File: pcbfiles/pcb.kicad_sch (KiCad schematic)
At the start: 236 parts, among them J1 Conn_01x06, J2 Conn_01x06, J3 Conn_01x06, J4 Conn_01x06, J5 Conn_01x04_Female, J6 Conn_01x04_Female, Q1 AO3401A, Q2 AO3401A, SW1 SW_SPST, SW10 SW_SPST, SW11 SW_SPST, SW12 SW_SPST, SW13 SW_SPST, SW14 SW_SPST, SW15 SW_SPST, SW16 SW_SPST, SW17 SW_SPST, SW18 SW_SPST, SW19 SW_SPST, SW2 SW_SPST, SW20 SW_SPST, SW21 SW_SPST, SW22 SW_SPST, SW23 SW_SPST, SW24 SW_SPST, SW25 SW_SPST, SW26 SW_SPST, SW27 SW_SPST, SW28 SW_SPST, SW29 SW_SPST, SW3 SW_SPST, SW30 SW_SPST, SW31 SW_SPST, SW32 SW_SPST, SW33 SW_SPST, SW34 SW_SPST, SW35 SW_SPST, SW36 SW_SPST, SW37 SW_SPST, SW38 SW_SPST, SW39 SW_SPST, SW4 SW_SPST, SW40 SW_SPST, SW41 SW_SPST, SW42 SW_SPST, SW43 SW_SPST, SW44 SW_SPST, SW45 SW_SPST, SW46 SW_SPST, SW47 SW_SPST, SW48 SW_SPST, SW49 SW_SPST, SW5 SW_SPST, SW50 SW_SPST, SW51 SW_SPST, SW52 SW_SPST, SW53 SW_SPST, SW54 SW_SPST, SW55 SW_SPST, SW56 SW_SPST, SW57 SW_SPST, SW58 SW_SPST, SW59 SW_SPST, SW6 SW_SPST, SW60 SW_SPST, SW61 SW_SPST, SW62 SW_SPST, SW63 SW_SPST, SW64 SW_SPST, SW65 SW_SPST, SW66 SW_SPST, SW67 SW_SPST, SW68 SW_SPST, SW69 SW_SPST, SW7 SW_SPST, SW70 SW_SPST, SW71 SW_SPST, SW72 SW_SPST, SW73 SW_SPST, SW74 SW_SPST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

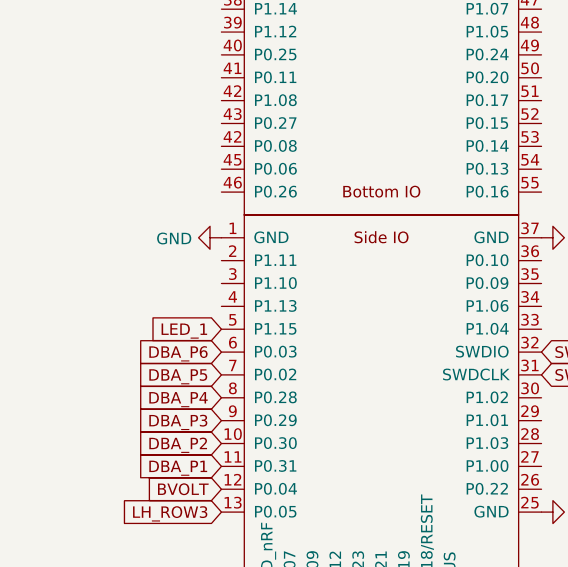
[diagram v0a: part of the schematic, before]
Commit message: Routing progress.
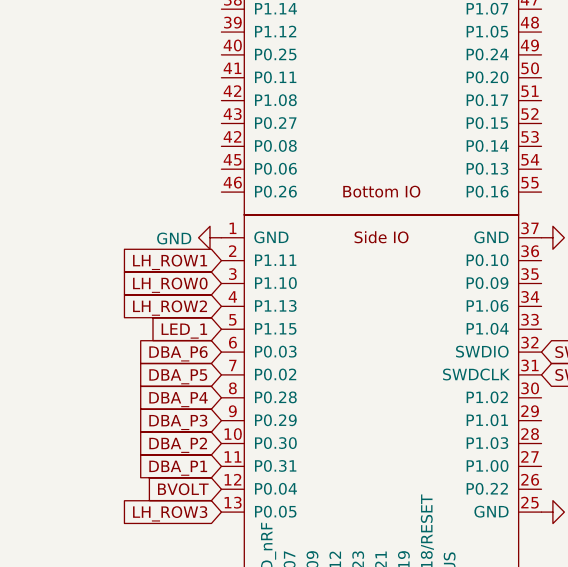
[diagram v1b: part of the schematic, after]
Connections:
- net LH_ROW0: now also U5.3 (P1.10)
- net LH_ROW1: now also U5.2 (P1.11)
- net LH_ROW2: now also U5.4 (P1.13)
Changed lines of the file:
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@@
+    )
+  )
+  (global_label "LH_ROW1" (shape input) (at 36.322 247.65 180) (fields_autoplaced)
+    (effects (font (size 1.27 1.27)) (justify right))
+    (property "Intersheet References" "${INTERSHEET_REFS}" (id 0) (at -90.678 124.46 0)
+      (effects (font (size 1.27 1.27)) hide)
     )
   )
@@
     )
   )
+  (global_label "LH_ROW0" (shape input) (at 36.322 250.19 180) (fields_autoplaced)
+    (effects (font (size 1.27 1.27)) (justify right))
+    (property "Intersheet References" "${INTERSHEET_REFS}" (id 0) (at -90.678 137.16 0)
+      (effects (font (size 1.27 1.27)) hide)
+    )
+  )
   (global_label "ENC_A_B" (shape input) (at 497.84 129.032 180) (fields_autoplaced)
     (effects (font (size 1.27 1.27)) (justify right))
@@
       (effects (font (size 1.27 1.27)) hide)
     )
+  )
+  (global_label "LH_ROW2" (shape input) (at 36.322 252.73 180) (fields_autoplaced)
+    (effects (font (size 1.27 1.27)) (justify right))
+    (property "Intersheet References" "${INTERSHEET_REFS}" (id 0) (at -90.678 119.38 0)
+      (effects (font (size 1.27 1.27)) hide)
+    )

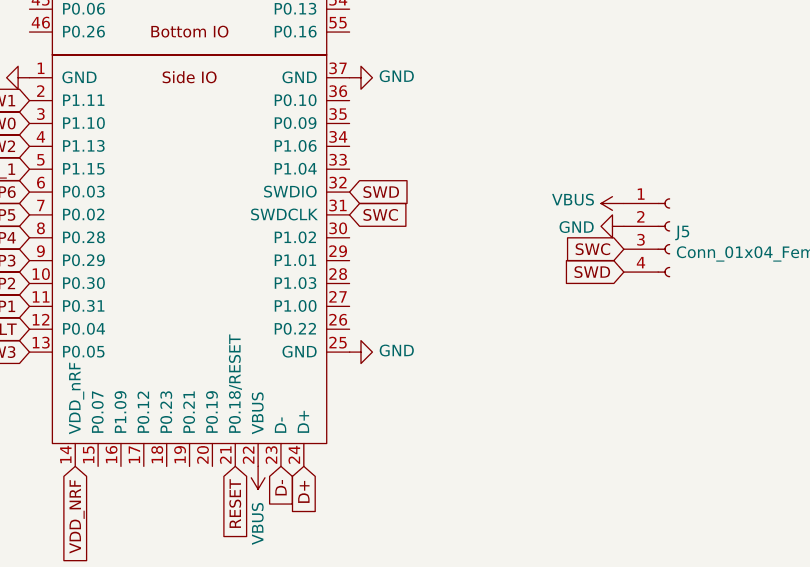
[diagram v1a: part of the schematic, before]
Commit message: practically done with the left half
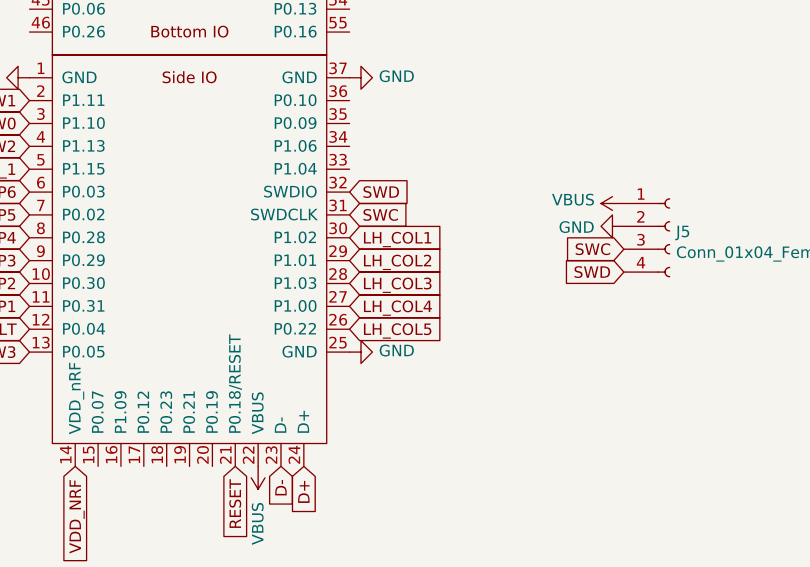
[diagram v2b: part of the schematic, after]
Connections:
- net LH_COL1: now also U5.30 (P1.02)
- net LH_COL2: now also U5.29 (P1.01)
- net LH_COL3: now also U5.28 (P1.03)
- net LH_COL4: now also U5.27 (P1.00)
- net LH_COL5: now also U5.26 (P0.22)
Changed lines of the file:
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@@
+    )
+  )
+  (global_label "LH_COL1" (shape input) (at 71.882 262.89 0) (fields_autoplaced)
+    (effects (font (size 1.27 1.27)) (justify left))
+    (property "Intersheet References" "${INTERSHEET_REFS}" (id 0) (at 169.672 110.49 0)
+      (effects (font (size 1.27 1.27)) hide)
     )
   )
@@
     )
   )
+  (global_label "LH_COL5" (shape input) (at 71.882 273.05 0) (fields_autoplaced)
+    (effects (font (size 1.27 1.27)) (justify left))
+    (property "Intersheet References" "${INTERSHEET_REFS}" (id 0) (at 169.672 49.53 0)
+      (effects (font (size 1.27 1.27)) hide)
+    )
+  )
   (global_label "LH_ROW0" (shape input) (at 36.322 250.19 180) (fields_autoplaced)
     (effects (font (size 1.27 1.27)) (justify right))
@@
     (effects (font (size 1.27 1.27)) (justify left))
     (property "Intersheet References" "${INTERSHEET_REFS}" (id 0) (at 30.988 160.274 0)
+      (effects (font (size 1.27 1.27)) hide)
+    )
+  )
+  (global_label "LH_COL3" (shape input) (at 71.882 267.97 0) (fields_autoplaced)
+    (effects (font (size 1.27 1.27)) (justify left))
+    (property "Intersheet References" "${INTERSHEET_REFS}" (id 0) (at 169.672 80.01 0)
       (effects (font (size 1.27 1.27)) hide)
     )
@@
     )
   )
+  (global_label "LH_COL4" (shape input) (at 71.882 270.51 0) (fields_autoplaced)
+    (effects (font (size 1.27 1.27)) (justify left))
+    (property "Intersheet References" "${INTERSHEET_REFS}" (id 0) (at 169.672 64.77 0)
+      (effects (font (size 1.27 1.27)) hide)
+    )
+  )
   (global_label "RH_ROW3" (shape input) (at 510.032 288.29 270) (fields_autoplaced)
     (effects (font (size 1.27 1.27)) (justify right))
@@
       (effects (font (size 1.27 1.27)) hide)
     )
+  )
+  (global_label "LH_COL2" (shape input) (at 71.882 265.43 0) (fields_autoplaced)
+    (effects (font (size 1.27 1.27)) (justify left))
+    (property "Intersheet References" "${INTERSHEET_REFS}" (id 0) (at 169.672 95.25 0)
+      (effects (font (size 1.27 1.27)) hide)
+    )

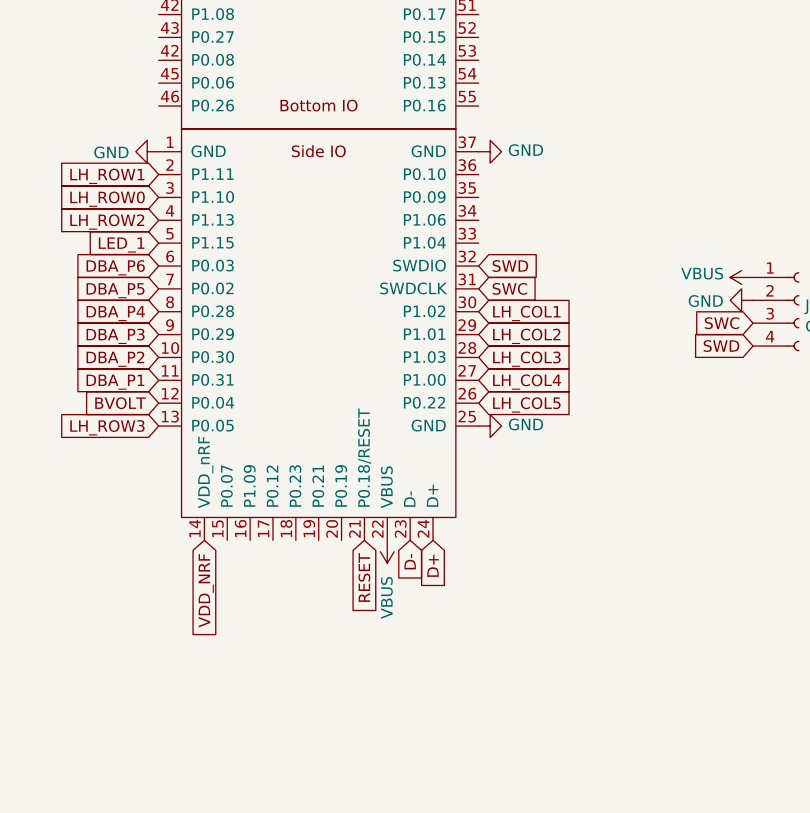
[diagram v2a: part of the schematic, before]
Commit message: Routing.
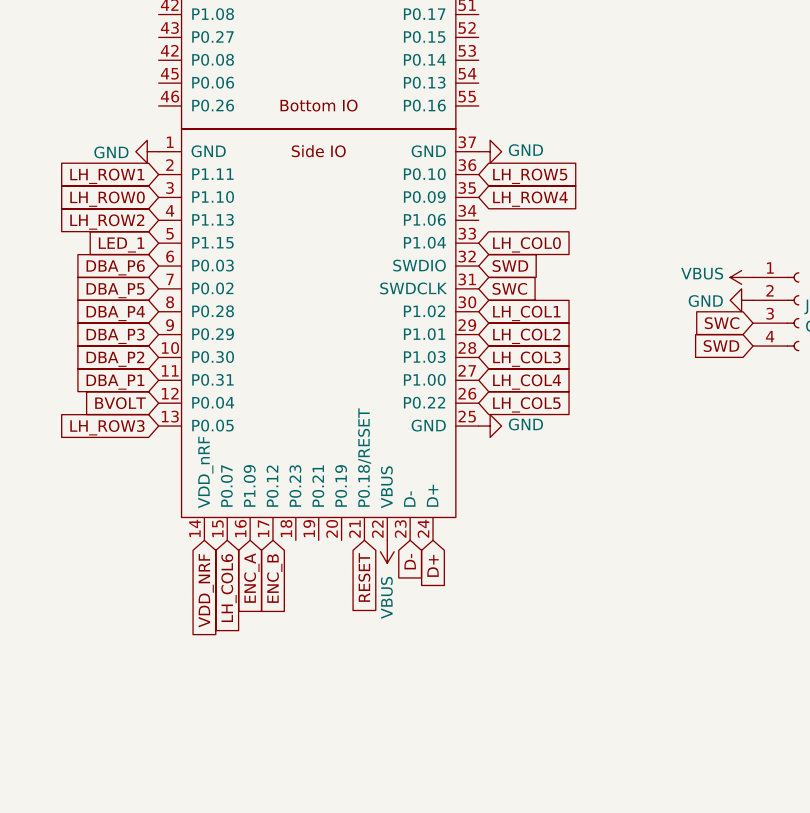
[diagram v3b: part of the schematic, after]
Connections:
- net ENC_A: now also U5.16 (P1.09)
- net ENC_B: now also U5.17 (P0.12)
- net ENC_P1: now also U5.15 (P0.07)
- net LH_COL0: now also U5.33 (P1.04)
- net LH_ROW4: now also U5.35 (P0.09)
- net LH_ROW5: now also U5.36 (P0.10)
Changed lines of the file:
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@@
+    )
+  )
+  (global_label "ENC_B" (shape input) (at 49.022 288.29 270) (fields_autoplaced)
+    (effects (font (size 1.27 1.27)) (justify right))
+    (property "Intersheet References" "${INTERSHEET_REFS}" (id 0) (at 49.1014 296.6013 90)
+      (effects (font (size 1.27 1.27)) (justify right) hide)
     )
   )
@@
     )
   )
+  (global_label "LH_ROW5" (shape input) (at 71.882 247.65 0) (fields_autoplaced)
+    (effects (font (size 1.27 1.27)) (justify left))
+    (property "Intersheet References" "${INTERSHEET_REFS}" (id 0) (at 198.882 411.48 0)
+      (effects (font (size 1.27 1.27)) hide)
+    )
+  )
+  (global_label "LH_COL0" (shape input) (at 71.882 255.27 0) (fields_autoplaced)
+    (effects (font (size 1.27 1.27)) (justify left))
+    (property "Intersheet References" "${INTERSHEET_REFS}" (id 0) (at 82.3705 255.1906 0)
+      (effects (font (size 1.27 1.27)) (justify left) hide)
+    )
+  )
   (global_label "DBA_P3" (shape input) (at 36.322 265.43 180) (fields_autoplaced)
     (effects (font (size 1.27 1.27)) (justify right))
@@
     )
   )
+  (global_label "ENC_A" (shape input) (at 46.482 288.29 270) (fields_autoplaced)
+    (effects (font (size 1.27 1.27)) (justify right))
+    (property "Intersheet References" "${INTERSHEET_REFS}" (id 0) (at 46.5614 296.4199 90)
+      (effects (font (size 1.27 1.27)) (justify right) hide)
+    )
+  )
   (global_label "VBUS_B" (shape input) (at 631.952 158.75 180) (fields_autoplaced)
     (effects (font (size 1.27 1.27)) (justify right))
     (property "Intersheet References" "${INTERSHEET_REFS}" (id 0) (at 60.452 128.27 0)
+      (effects (font (size 1.27 1.27)) hide)
+    )
+  )
+  (global_label "LH_ROW4" (shape input) (at 71.882 250.19 0) (fields_autoplaced)
+    (effects (font (size 1.27 1.27)) (justify left))
+    (property "Intersheet References" "${INTERSHEET_REFS}" (id 0) (at 198.882 403.86 0)
       (effects (font (size 1.27 1.27)) hide)
     )
@@
       (effects (font (size 1.27 1.27)) hide)
     )
+  )
+  (global_label "LH_COL6" (shape input) (at 43.942 288.29 270) (fields_autoplaced)
+    (effects (font (size 1.27 1.27)) (justify right))
+    (property "Intersheet References" "${INTERSHEET_REFS}" (id 0) (at 285.242 386.08 0)
+      (effects (font (size 1.27 1.27)) hide)
+    )

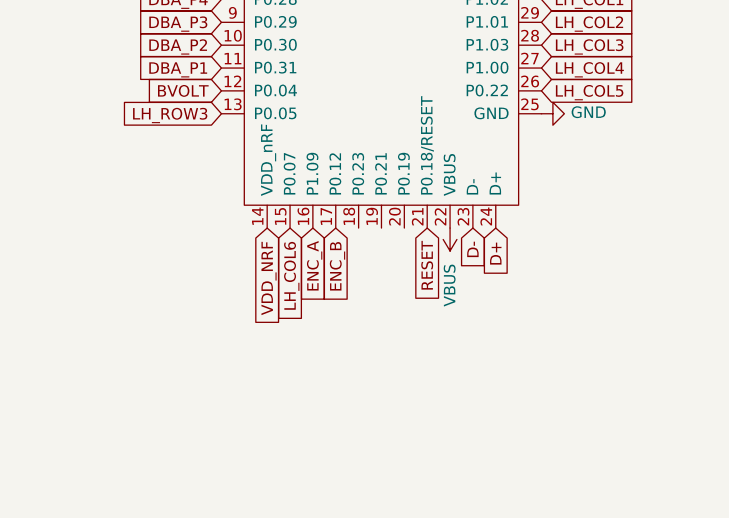
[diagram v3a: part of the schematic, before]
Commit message: Routing.
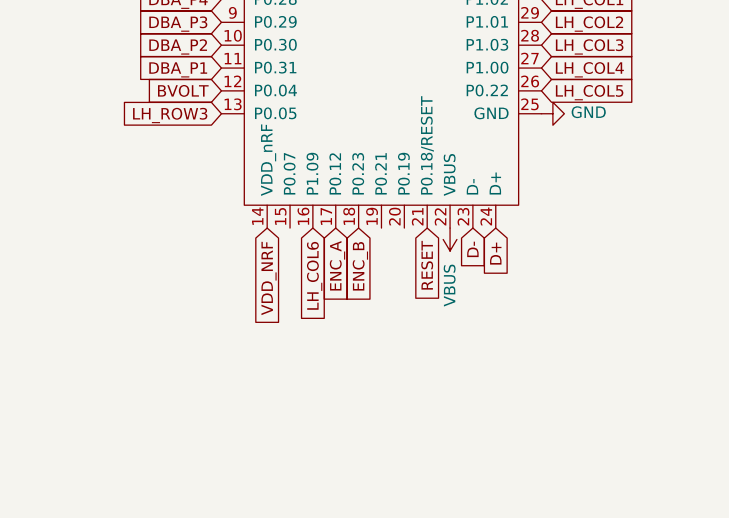
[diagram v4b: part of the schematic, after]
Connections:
- net ENC_A: now also U5.17 (P0.12); no longer U5.16 (P1.09)
- net ENC_B: now also U5.18 (P0.23); no longer U5.17 (P0.12)
- net ENC_P1: now also U5.16 (P1.09); no longer U5.15 (P0.07)
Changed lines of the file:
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@@
     )
   )
-  (global_label "ENC_B" (shape input) (at 49.022 288.29 270) (fields_autoplaced)
-    (effects (font (size 1.27 1.27)) (justify right))
-    (property "Intersheet References" "${INTERSHEET_REFS}" (id 0) (at 49.1014 296.6013 90)
+  (global_label "ENC_B" (shape input) (at 51.562 288.29 270) (fields_autoplaced)
+    (effects (font (size 1.27 1.27)) (justify right))
+    (property "Intersheet References" "${INTERSHEET_REFS}" (id 0) (at 51.6414 296.6013 90)
       (effects (font (size 1.27 1.27)) (justify right) hide)
     )
@@
     )
   )
-  (global_label "ENC_A" (shape input) (at 46.482 288.29 270) (fields_autoplaced)
-    (effects (font (size 1.27 1.27)) (justify right))
-    (property "Intersheet References" "${INTERSHEET_REFS}" (id 0) (at 46.5614 296.4199 90)
+  (global_label "ENC_A" (shape input) (at 49.022 288.29 270) (fields_autoplaced)
+    (effects (font (size 1.27 1.27)) (justify right))
+    (property "Intersheet References" "${INTERSHEET_REFS}" (id 0) (at 49.1014 296.4199 90)
       (effects (font (size 1.27 1.27)) (justify right) hide)
     )
@@
     )
   )
-  (global_label "LH_COL6" (shape input) (at 43.942 288.29 270) (fields_autoplaced)
-    (effects (font (size 1.27 1.27)) (justify right))
-    (property "Intersheet References" "${INTERSHEET_REFS}" (id 0) (at 285.242 386.08 0)
-      (effects (font (size 1.27 1.27)) hide)
-    )
+  (global_label "LH_COL6" (shape input) (at 46.482 288.29 270) (fields_autoplaced)
+    (effects (font (size 1.27 1.27)) (justify right))
+    (property "Intersheet References" "${INTERSHEET_REFS}" (id 0) (at 287.782 386.08 0)
+      (effects (font (size 1.27 1.27)) hide)
+    )

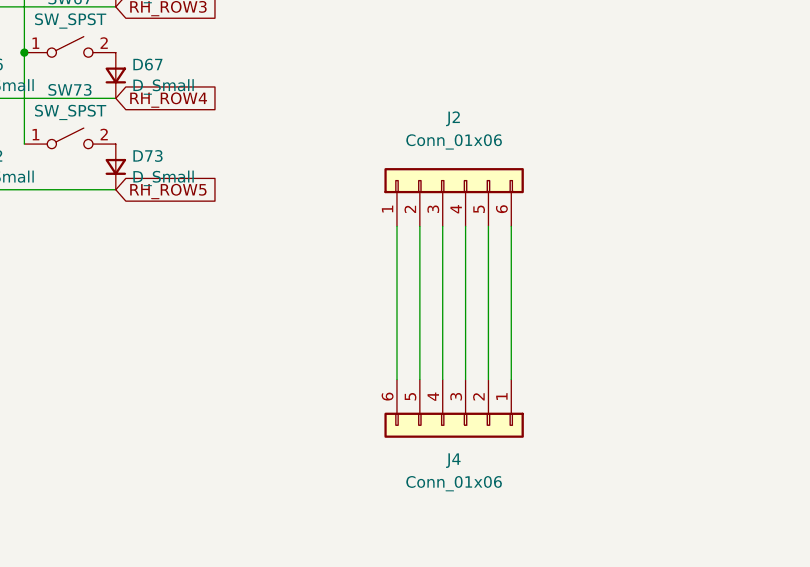
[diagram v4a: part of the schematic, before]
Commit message: Routing.
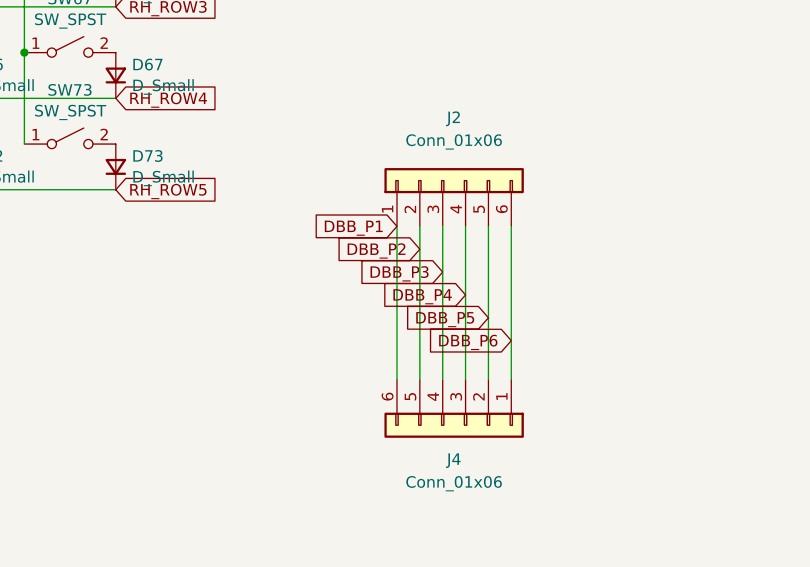
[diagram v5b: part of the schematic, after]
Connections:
- net DBB_P1: now reaches J2.1 (Pin_1), J4.6 (Pin_6)
- net DBB_P2: now reaches J2.2 (Pin_2), J4.5 (Pin_5)
- net DBB_P3: now reaches J2.3 (Pin_3), J4.4 (Pin_4)
- net DBB_P4: now reaches J2.4 (Pin_4), J4.3 (Pin_3)
- net DBB_P5: now reaches J2.5 (Pin_5), J4.2 (Pin_2)
- net DBB_P6: now reaches J2.6 (Pin_6), J4.1 (Pin_1)
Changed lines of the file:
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@@
+    )
+  )
+  (global_label "DBB_P3" (shape input) (at 636.524 100.838 180) (fields_autoplaced)
+    (effects (font (size 1.27 1.27)) (justify right))
+    (property "Intersheet References" "${INTERSHEET_REFS}" (id 0) (at 626.9427 100.7586 0)
+      (effects (font (size 1.27 1.27)) (justify right) hide)
     )
   )
@@
     )
   )
+  (global_label "DBB_P6" (shape input) (at 644.144 108.458 180) (fields_autoplaced)
+    (effects (font (size 1.27 1.27)) (justify right))
+    (property "Intersheet References" "${INTERSHEET_REFS}" (id 0) (at 634.5627 108.3786 0)
+      (effects (font (size 1.27 1.27)) (justify right) hide)
+    )
+  )
   (global_label "ENC_B" (shape input) (at 51.562 288.29 270) (fields_autoplaced)
     (effects (font (size 1.27 1.27)) (justify right))
@@
     )
   )
+  (global_label "DBB_P4" (shape input) (at 639.064 103.378 180) (fields_autoplaced)
+    (effects (font (size 1.27 1.27)) (justify right))
+    (property "Intersheet References" "${INTERSHEET_REFS}" (id 0) (at 629.4827 103.2986 0)
+      (effects (font (size 1.27 1.27)) (justify right) hide)
+    )
+  )
   (global_label "RAW" (shape input) (at 111.252 153.67 180) (fields_autoplaced)
     (effects (font (size 1.27 1.27)) (justify right))
@@
     )
   )
+  (global_label "DBB_P5" (shape input) (at 641.604 105.918 180) (fields_autoplaced)
+    (effects (font (size 1.27 1.27)) (justify right))
+    (property "Intersheet References" "${INTERSHEET_REFS}" (id 0) (at 632.0227 105.8386 0)
+      (effects (font (size 1.27 1.27)) (justify right) hide)
+    )
+  )
   (global_label "RH_COL4" (shape input) (at 554.482 25.654 90) (fields_autoplaced)
     (effects (font (size 1.27 1.27)) (justify left))
@@
     )
   )
+  (global_label "DBB_P1" (shape input) (at 631.444 95.758 180) (fields_autoplaced)
+    (effects (font (size 1.27 1.27)) (justify right))
+    (property "Intersheet References" "${INTERSHEET_REFS}" (id 0) (at 621.8627 95.6786 0)
+      (effects (font (size 1.27 1.27)) (justify right) hide)
+    )
+  )
   (global_label "SWD_B" (shape input) (at 555.752 266.7 180) (fields_autoplaced)
     (effects (font (size 1.27 1.27)) (justify right))
@@
     )
   )
+  (global_label "DBB_P2" (shape input) (at 633.984 98.298 180) (fields_autoplaced)
+    (effects (font (size 1.27 1.27)) (justify right))
+    (property "Intersheet References" "${INTERSHEET_REFS}" (id 0) (at 624.4027 98.2186 0)
+      (effects (font (size 1.27 1.27)) (justify right) hide)
+    )
+  )
